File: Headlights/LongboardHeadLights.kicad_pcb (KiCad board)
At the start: 2 copper layers, 76.2 x 10.8 mm, 16 parts, among them P1 CONN_01X03, U1 AL8805

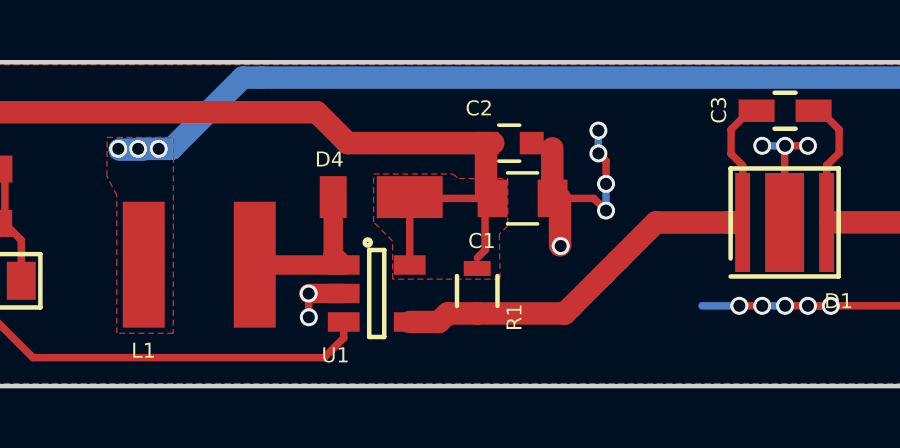
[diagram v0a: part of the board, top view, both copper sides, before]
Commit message: yet another fix
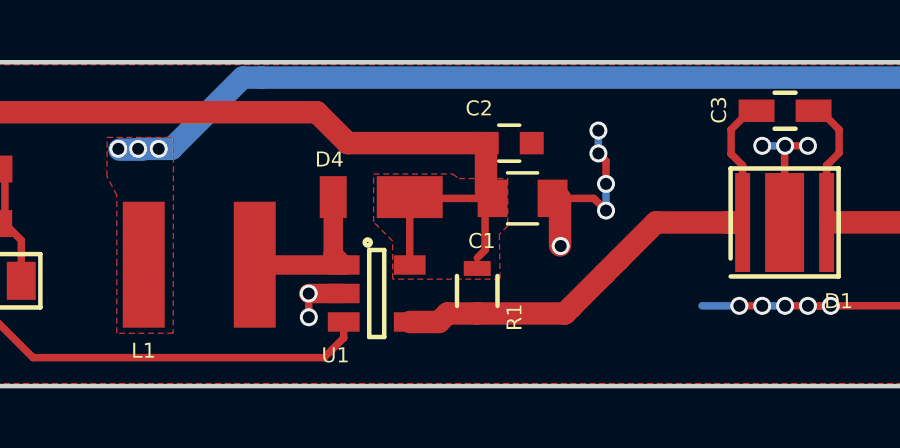
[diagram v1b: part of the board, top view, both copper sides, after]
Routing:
- net GND: track 62.9 -> 61.6 mm
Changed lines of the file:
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@@
     (thickness 1.6)
     (drawings 9)
-    (tracks 180)
+    (tracks 179)
     (zones 0)
     (modules 16)
@@
   (page A4)
   (layers
-    (0 F.Cu signal hide)
-    (31 B.Cu signal)
+    (0 F.Cu signal)
+    (31 B.Cu signal hide)
     (32 B.Adhes user)
     (33 F.Adhes user)
@@
   (segment (start 134.4682 87.7824) (end 134.195849 88.054751) (width 0.75) (layer F.Cu) (net 1))
   (segment (start 149.2504 88.8111) (end 148.2217 87.7824) (width 0.75) (layer F.Cu) (net 1))
-  (segment (start 154.1043 88.8111) (end 149.2504 88.8111) (width 0.75) (layer F.Cu) (net 1))
+  (segment (start 153.75 88.8111) (end 149.2504 88.8111) (width 0.75) (layer F.Cu) (net 1))
   (segment (start 134.195849 88.054751) (end 134.195849 88.054151) (width 0.25) (layer F.Cu) (net 1))
   (segment (start 133.3627 90.8939) (end 133.3627 88.8879) (width 0.75) (layer F.Cu) (net 1))
@@
   (segment (start 156.3297 92.2201) (end 156.3497 92.2401) (width 0.25) (layer F.Cu) (net 2))
   (via (at 156.3497 92.2401) (size 0.6) (drill 0.4) (layers F.Cu B.Cu) (net 2))
-  (segment (start 156.0703 88.9841) (end 156.0703 90.297) (width 0.75) (layer F.Cu) (net 2))
   (segment (start 149.117764 93.823146) (end 147.951854 93.823146) (width 0.65) (layer F.Cu) (net 2))
   (segment (start 147.951854 93.823146) (end 147.95 93.825) (width 0.25) (layer F.Cu) (net 2))
